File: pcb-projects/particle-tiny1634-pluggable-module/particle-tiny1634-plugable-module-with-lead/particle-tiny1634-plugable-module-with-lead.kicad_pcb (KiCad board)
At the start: 2 copper layers, 37.5 x 47.6 mm, 33 parts, among them IC1 ATTINY1634-SU, P1 INTERFACE, P2 MCU_TEST

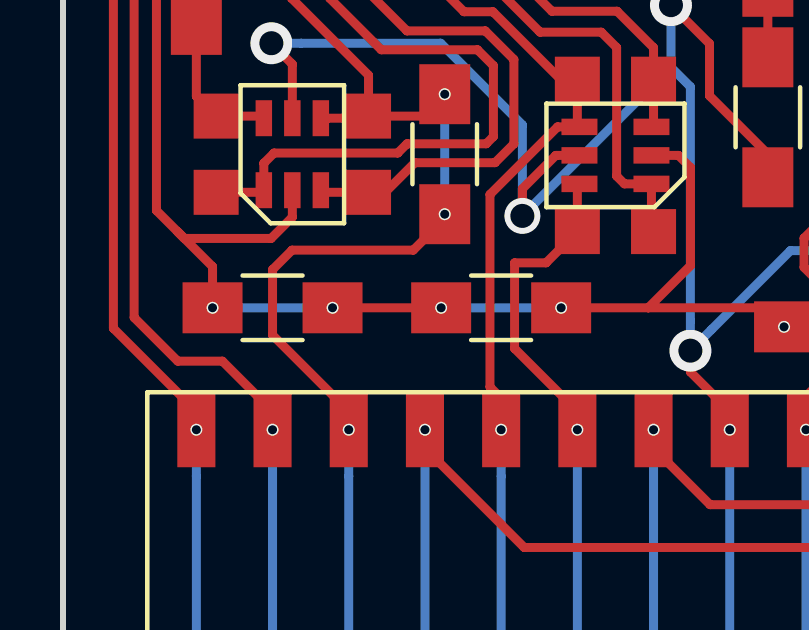
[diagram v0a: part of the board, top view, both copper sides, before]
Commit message: cleanup folders; minimal pcb changes
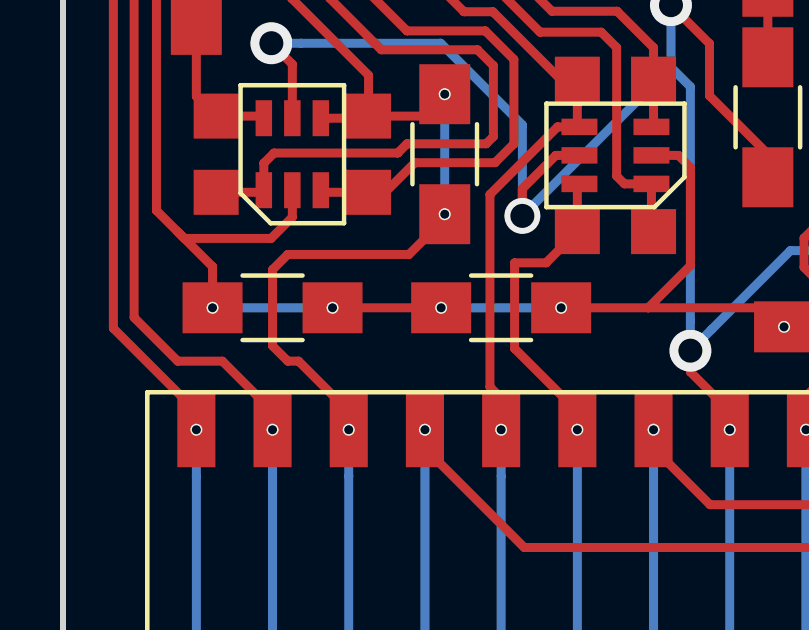
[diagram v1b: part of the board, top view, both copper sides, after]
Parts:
- renumbered Q-CHAIN1 to Q-EAST1
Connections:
- net /PWR/TX-CHAIN renamed /SW_PWR_TX-EAST
- net /PWR/TX-NORTH renamed /SW_PWR_TX-NORTH
- net /PWR/TX-SOUTH renamed /SW_PWR_TX-SOUTH
- net /RX-CHAIN renamed /RX-EAST
- net /SW_PWR/RX-CHAIN renamed /SW_PWR_RX-EAST
- net /SW_PWR/RX-NORTH renamed /SW_PWR_RX-NORTH
- net /SW_PWR/RX-SOUTH renamed /SW_PWR_RX-SOUTH
- net /TX-CHAIN renamed /TX-EAST
